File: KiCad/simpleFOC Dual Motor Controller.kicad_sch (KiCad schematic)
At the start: 25 parts, among them J101 Conn_01x04, J102 USB_C_Receptacle_USB2.0_14P, J103 Conn_01x06, J104 Conn_01x06, SW101 TS-1088-AR02016, U101 XC6206P332MR, U102 XT60H-M, U103 ESP32-S3-WROOM-1, U104 H5VND5UB

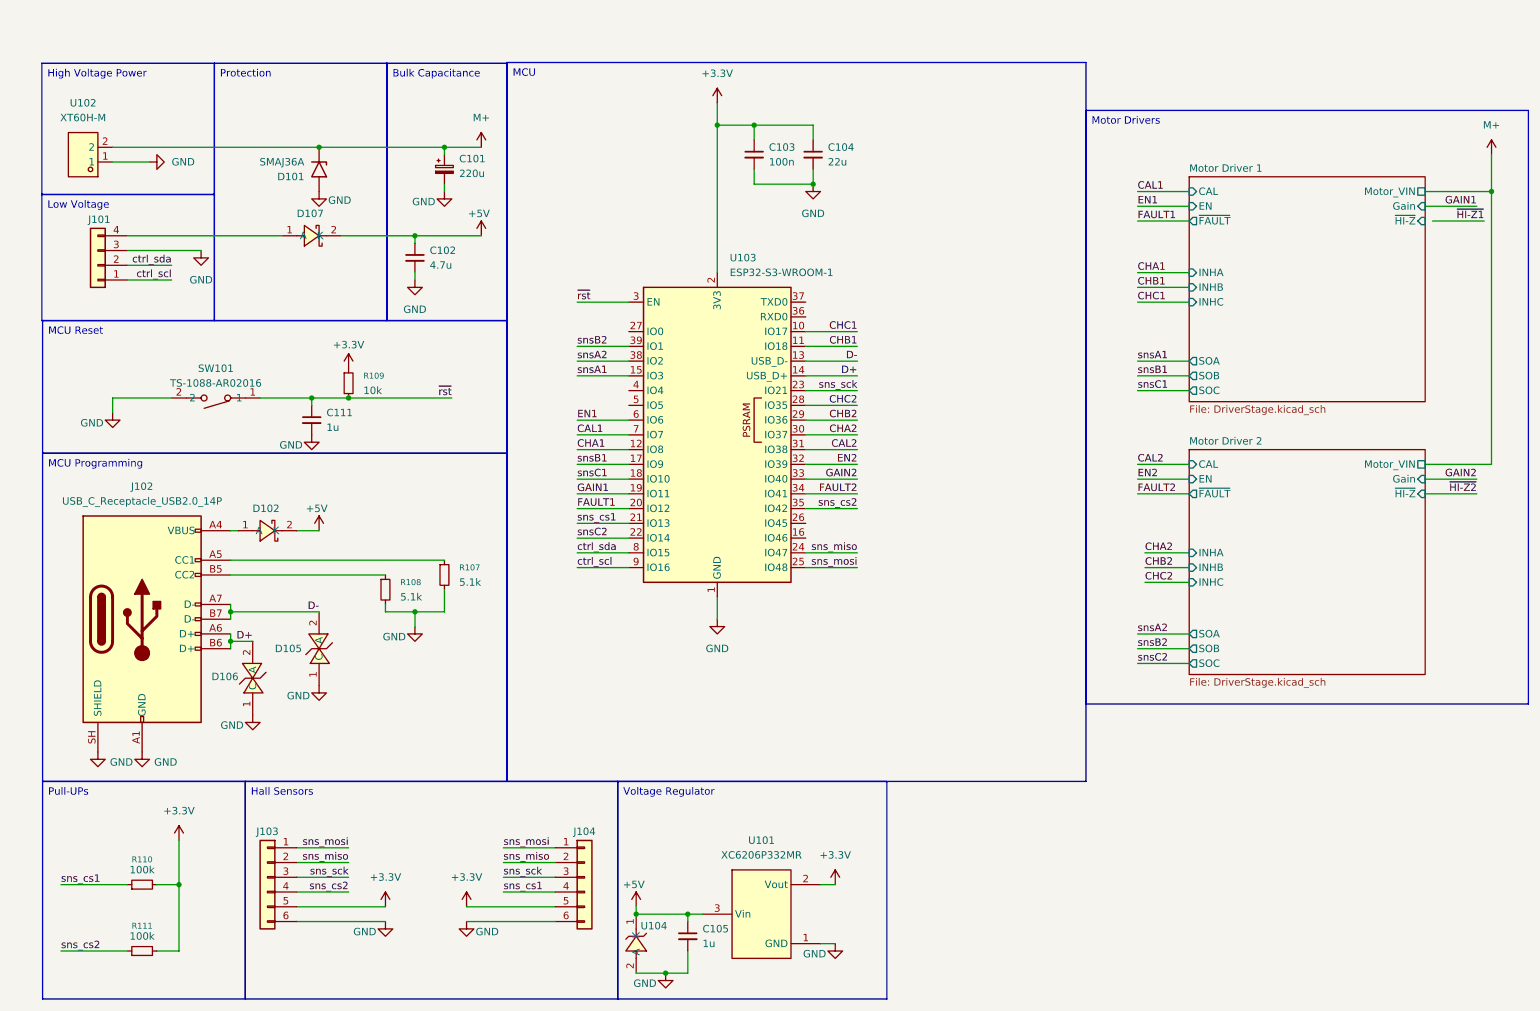
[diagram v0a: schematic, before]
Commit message: finished iteration 1
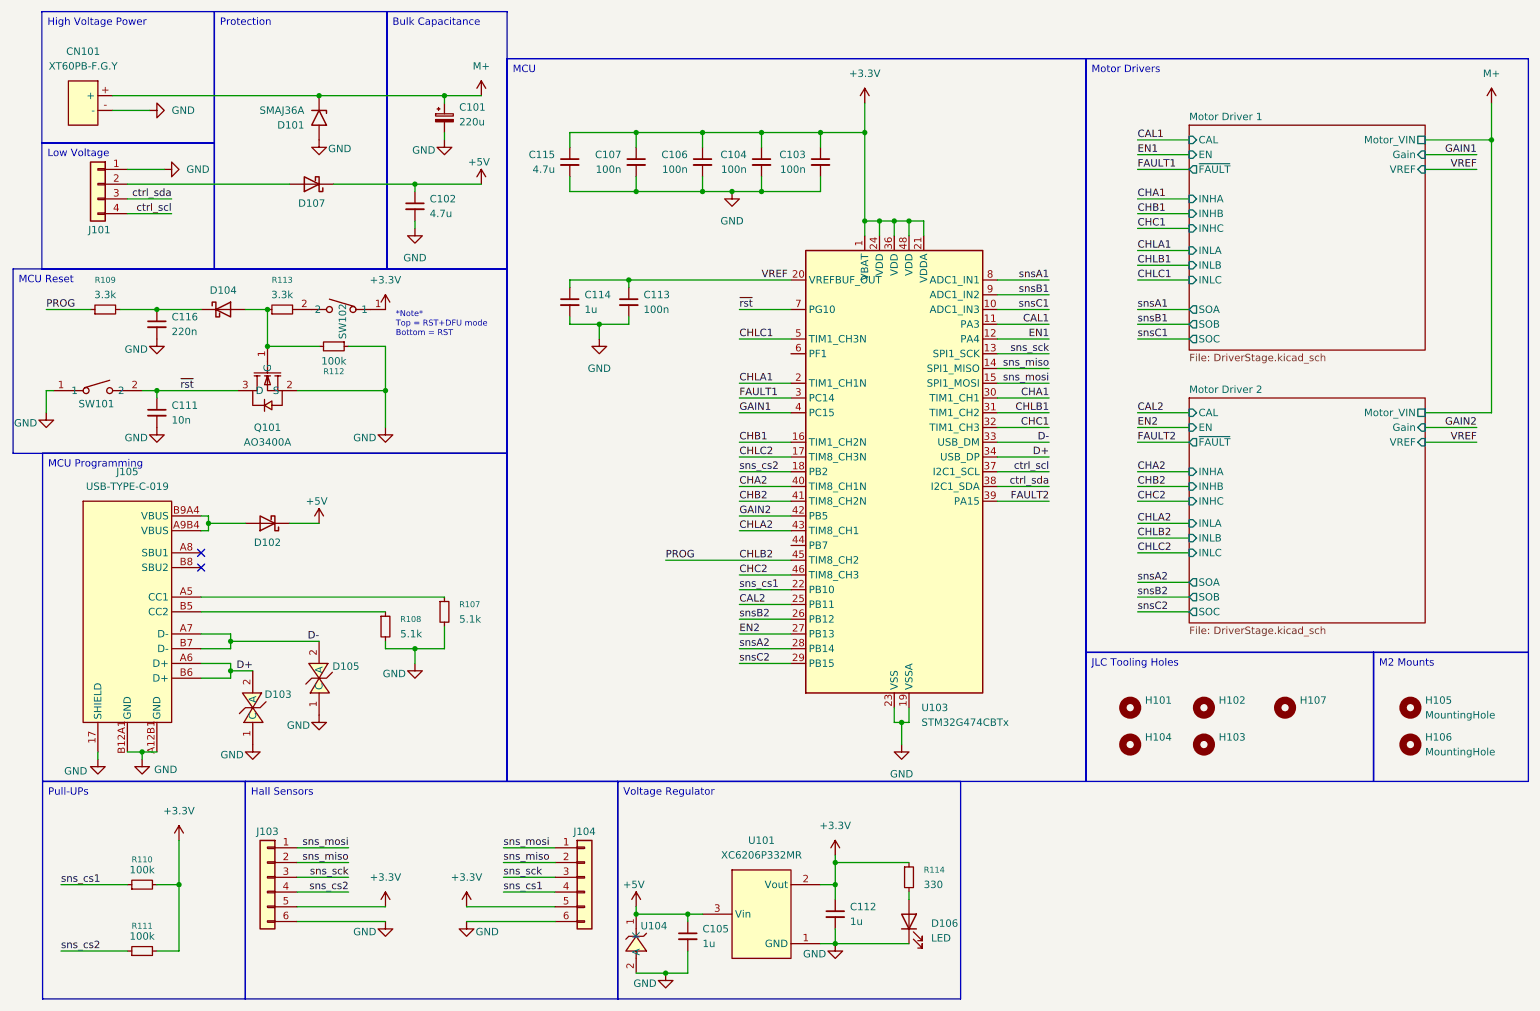
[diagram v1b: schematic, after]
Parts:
- removed D102, D107: B16WS_C7420327, easyeda2kicad:SOD-323_L1.7-W1.3-LS2.5-FD, symbol easyeda2kicad:B16WS_C7420327
- removed D105, D106: H5VL06B, easyeda2kicad:X3-DFN0603-2_L0.6-W0.3-BI, symbol easyeda2kicad:H5VL06B
- removed J102: USB_C_Receptacle_USB2.0_14P, Connector_USB:USB_C_Receptacle_HCTL_HC-TYPE-C-16P-01A, symbol Connector:USB_C_Receptacle_USB2.0_14P
- removed U102: XT60H-M, easyeda2kicad:CONN-TH_XT60H-M, symbol easyeda2kicad:XT60H-M
- removed U103: ESP32-S3-WROOM-1, RF_Module:ESP32-S3-WROOM-1, symbol RF_Module:ESP32-S3-WROOM-1
- added C106, C107, C113: 100n, Capacitor_SMD:C_0402_1005Metric, symbol Device:C_Small
- added C112, C114: 1u, Capacitor_SMD:C_0402_1005Metric, symbol Device:C_Small
- added C115: 4.7u, Capacitor_SMD:C_0402_1005Metric, symbol Device:C_Small
- added C116: 220n, Capacitor_SMD:C_0402_1005Metric, symbol Device:C_Small
- added CN101: XT60PB-F.G.Y, easyeda2kicad:CONN-TH_XT60PB-F.G.Y, symbol easyeda2kicad:XT60PB-F.G.Y
- added D102, D104, D107: 1N5819WS, Diode_SMD:D_SOD-323, symbol Diode:1N5819WS
- added D103, D105: H5VL10B, easyeda2kicad:SOD-882_L1.0-W0.6-BI, symbol easyeda2kicad:H5VL10B
- added D106: LED, LED_SMD:LED_0603_1608Metric, symbol Device:LED
- added H101, H102, H103, H104, H107: MountingHole, easyeda2kicad:JLC_Tooling_Hole, symbol Mechanical:MountingHole
- added H105, H106: MountingHole, MountingHole:MountingHole_2.2mm_M2, symbol Mechanical:MountingHole
- added J105: USB-TYPE-C-019, easyeda2kicad:TYPE-C-SMD_HX-TYPE-C-16PIN, symbol easyeda2kicad:USB-TYPE-C-019
- added Q101: AO3400A, easyeda2kicad:SOT-23-3_L2.9-W1.3-P1.90-LS2.4-BR, symbol easyeda2kicad:AO3400A
- added R112: 100k, Resistor_SMD:R_0402_1005Metric, symbol Device:R_Small
- added R113: 3.3k, PCM_SparkFun-Resistor:R_0402_1005Metric, symbol Device:R_Small
- added R114: 330, Resistor_SMD:R_0402_1005Metric, symbol Device:R_Small
- added SW102: TS-1088-AR02016, easyeda2kicad:SW-SMD_L3.9-W3.0-P4.45, symbol easyeda2kicad:TS-1088-AR02016
- added U103: STM32G474CBTx, Package_QFP:LQFP-48_7x7mm_P0.5mm, symbol MCU_ST_STM32G4:STM32G474CBTx
- C102: footprint (none) -> Capacitor_SMD:C_0402_1005Metric
- C104: value 22u -> 100n; footprint Capacitor_SMD:C_0603_1608Metric -> Capacitor_SMD:C_0402_1005Metric
- C111: value 1u -> 10n
- R109: value 10k -> 3.3k
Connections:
- net +3.3V: now also C106.1, C107.1, C112.1, C115.1, R114.1, SW102.1, U103.1 (VBAT), U103.21 (VDDA), U103.24 (VDD), U103.36 (VDD), U103.48 (VDD); no longer R109.1
- net +5V: now also D102.1 (K), D107.1 (K)
- net CAL1: now also U103.11 (PA3)
- net CAL2: now also U103.25 (PB11)
- net CHA1: now also U103.30 (PA8)
- net CHA2: now also U103.40 (PB3)
- net CHB1: now also U103.16 (PB0)
- net CHB2: now also U103.41 (PB4)
- net CHC1: now also U103.32 (PA10)
- net CHC2: now also U103.46 (PB9)
- net D+: now also D103.2 (A), J105.A6 (D+), J105.B6 (D+), U103.34 (PA12)
- net D-: now also D105.2 (A), J105.A7 (D-), J105.B7 (D-), U103.33 (PA11)
- net EN1: now also U103.12 (PA4)
- net EN2: now also U103.27 (PB13)
- net FAULT1: now also U103.3 (PC14)
- net FAULT2: now also U103.39 (PA15)
- net GAIN1: now also U103.4 (PC15)
- net GAIN2: now also U103.42 (PB5)
- net GND: now also J101.1 (Pin_1), SW101.1, C106.2, C107.2, C112.2, C113.2, C114.2, C115.2, C116.2, CN101.-, D103.1 (C), D105.1 (C), D106.1 (K), J105.17 (SHIELD), J105.A12B1 (GND), J105.B12A1 (GND), Q101.2 (S), R112.1, U103.19 (VSSA), U103.23 (VSS), U103.35 (VSS), U103.47 (VSS); no longer J101.3 (Pin_3), SW101.2
- net M+: now also CN101.+
- net ctrl_scl: now also J101.4 (Pin_4), U103.37 (PA13); no longer J101.1 (Pin_1)
- net ctrl_sda: now also J101.3 (Pin_3), U103.38 (PA14); no longer J101.2 (Pin_2)
- net snsA1: now also U103.8 (PA0)
- net snsA2: now also U103.28 (PB14)
- net snsB1: now also U103.9 (PA1)
- net snsB2: now also U103.26 (PB12)
- net snsC1: now also U103.10 (PA2)
- net snsC2: now also U103.29 (PB15)
- net sns_cs1: now also U103.22 (PB10)
- net sns_cs2: now also U103.18 (PB2)
- net sns_miso: now also U103.14 (PA6)
- net sns_mosi: now also U103.15 (PA7)
- net sns_sck: now also U103.13 (PA5)
- net ~{rst}: now also SW101.2, Q101.3 (D), U103.7 (PG10); no longer R109.2, SW101.1
- net at R108.1: now also J105.B5 (CC2)
- net at R107.1: now also J105.A5 (CC1)
- new net: C116.1, D104.1 (K), R109.2
- new net: D104.2 (A), Q101.1 (G), R112.2, R113.1
- new net: D102.2 (A), J105.A9B4 (VBUS), J105.B9A4 (VBUS)
- new net: R113.2, SW102.2
- new net: D106.2 (A), R114.2
- new net: D107.2 (A), J101.2 (Pin_2)
- new net CHLA1: U103.2 (PC13)
- new net CHLA2: U103.43 (PB6)
- new net CHLB1: U103.31 (PA9)
- new net CHLB2: R109.1, U103.45 (PB8)
- new net CHLC1: U103.5 (PF0)
- new net CHLC2: U103.17 (PB1)
- new net VREF: C113.1, C114.1, U103.20 (VREF+)
- no-connect marks 0 -> 2
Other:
- sheet Motor Driver 1 ports: added INLA, INLB, INLC, VREF; removed ~{HI-Z}
- sheet Motor Driver 2 ports: added INLA, INLB, INLC, VREF; removed ~{HI-Z}
- note added: "*Note* Top = RST+DFU mode Bottom = RST"
- moved on the sheet: C101, C102, C111, D101, R107, R108, SW101
